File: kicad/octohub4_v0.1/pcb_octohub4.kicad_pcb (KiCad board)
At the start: 2 copper layers, 100 x 80 mm, 85 parts, among them J101 USB231ARY, J102 USB231ARY, J103 USB231ARY, J104 USB231ARY, J201 Screw_Terminal_01x02, J203 Barrel_Jack_Switch, J301 USB_C_Receptacle_USB2.0, U201 TPS259474LRPWR, U301 AMS1117-3.3, U302 USB2514B_Bi, Y301 24MHz

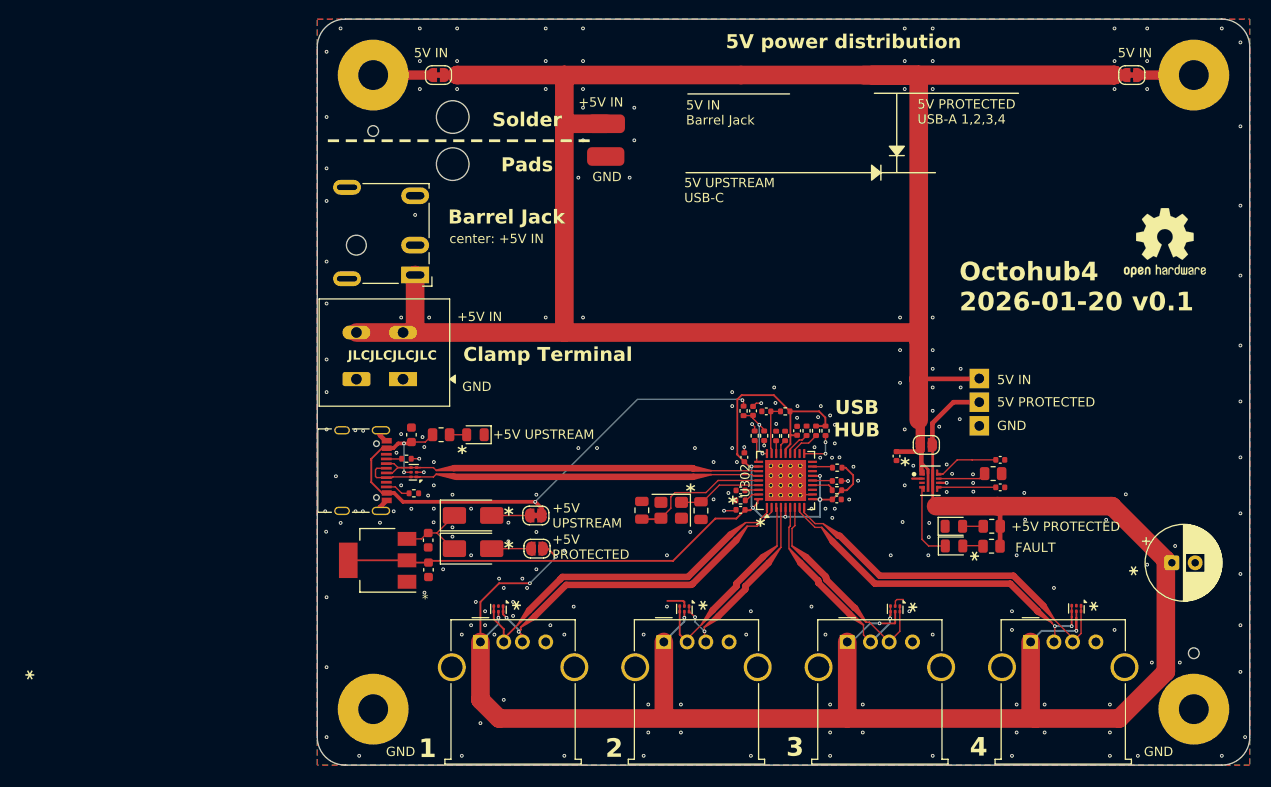
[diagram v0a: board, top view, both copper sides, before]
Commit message: Version v0.1. Manually fix all violations.
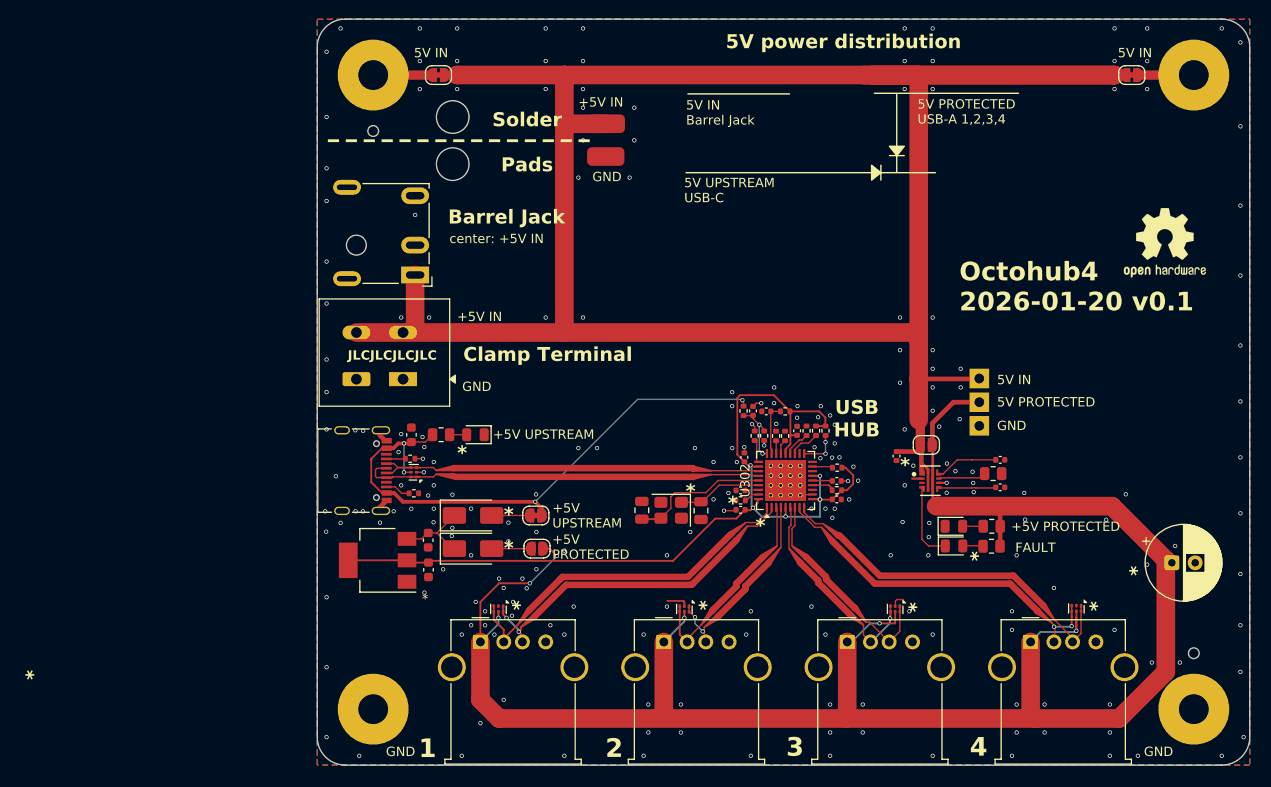
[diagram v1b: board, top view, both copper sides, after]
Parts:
- moved R302 0.39 mm to (68.7, 64.4)
